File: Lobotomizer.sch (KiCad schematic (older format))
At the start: 3 parts, among them J1 IN, J2 OUT, J3 Barrel_Jack

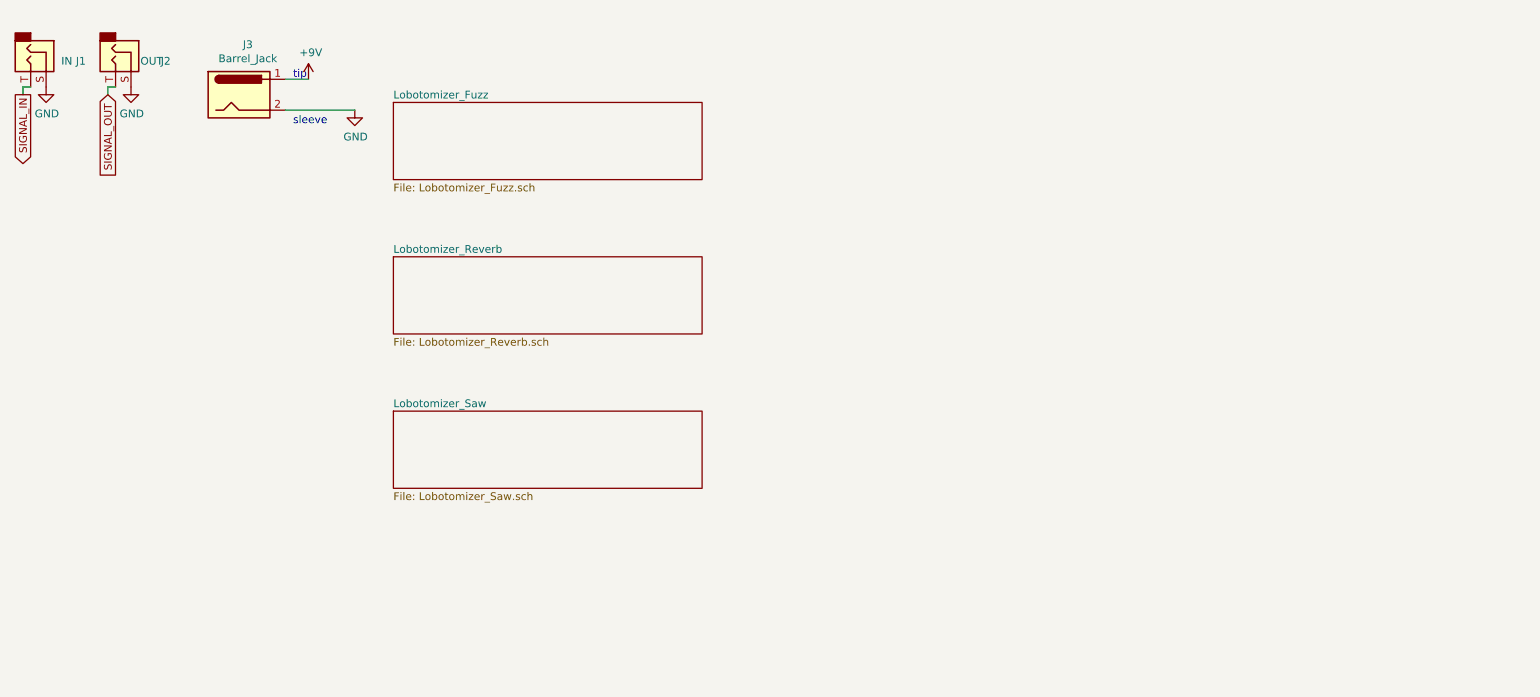
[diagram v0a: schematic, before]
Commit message: lobotomizer v2 update
so much changed i cant note it all here
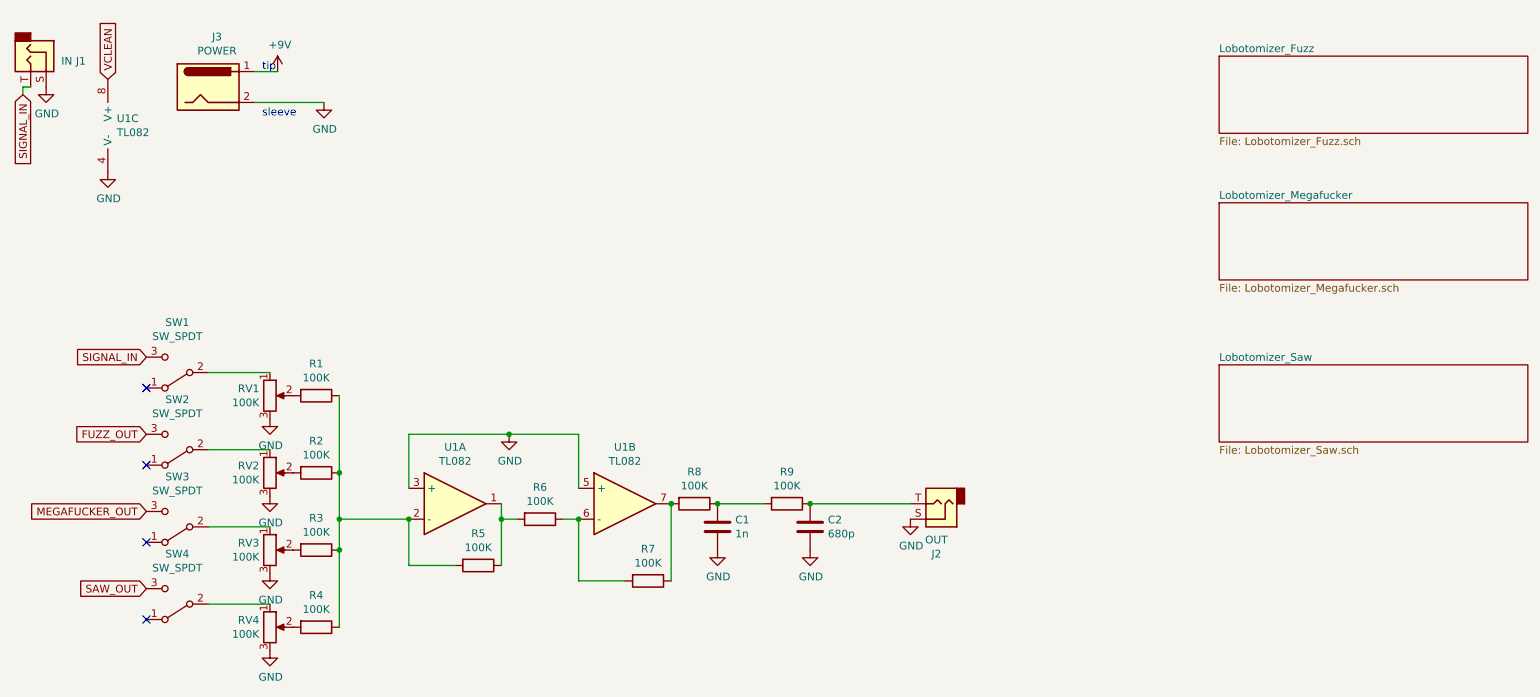
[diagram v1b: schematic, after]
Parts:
- added C1: 1n, Capacitor_THT:C_Disc_D3.8mm_W2.6mm_P2.50mm, symbol Device:C
- added C2: 680p, Capacitor_THT:C_Disc_D4.3mm_W1.9mm_P5.00mm, symbol Device:C
- added R1, R2, R3, R4, R5, R6, R7, R8, R9: 100K, Resistor_THT:R_Axial_DIN0204_L3.6mm_D1.6mm_P5.08mm_Horizontal, symbol Device:R
- added RV1, RV2, RV3, RV4: 100K, Potentiometer_THT:Potentiometer_Bourns_3266Y_Vertical, symbol Device:R_POT
- added SW1, SW2, SW3, SW4: SW_SPDT, TerminalBlock_Phoenix:TerminalBlock_Phoenix_MKDS-1,5-3-5.08_1x03_P5.08mm_Horizontal, symbol Switch:SW_SPDT
- added U1: TL082, Package_DIP:DIP-8_W7.62mm, symbol Device:Opamp_Dual_Generic
- J1, J2: footprint Connector_Audio:Jack_6.35mm_Neutrik_NMJ4HCD2_Horizontal -> Connector_Audio:Jack_6.35mm_Neutrik_NMJ4HFD2_Horizontal
- J3: value Barrel_Jack -> POWER; footprint Connector_BarrelJack:BarrelJack_Horizontal -> Connector_BarrelJack:BarrelJack_CUI_PJ-063AH_Horizontal
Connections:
- net GND: now also C1.2, C2.2, RV1.3, RV2.3, RV3.3, RV4.3, U1.3 (+), U1.4 (V-), U1.5 (+)
- net SIGNAL_IN: now also SW1.3 (C)
- net SIGNAL_OUT: no longer names the net of J2.T
- net SIGNAL_OUT: now also C2.1, R9.1
- new net: RV3.1, SW3.2 (B)
- new net: RV2.1, SW2.2 (B)
- new net: RV1.1, SW1.2 (B)
- new net: RV4.1, SW4.2 (B)
- new net: R1.2, RV1.2
- new net: R2.2, RV2.2
- new net: R3.2, RV3.2
- new net: R4.2, RV4.2
- new net: R1.1, R2.1, R3.1, R4.1, R5.2, U1.2 (-)
- new net: R5.1, R6.2, U1.1
- new net: R6.1, R7.2, U1.6 (-)
- new net: R7.1, R8.2, U1.7
- new net: C1.1, R8.1, R9.2
- new net FUZZ_OUT: SW2.3 (C)
- new net MEGAFUCKER_OUT: SW3.3 (C)
- new net SAW_OUT: SW4.3 (C)
- new net VCLEAN: U1.8 (V+)
- no-connect marks 0 -> 4
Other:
- moved on the sheet: J2, J3
